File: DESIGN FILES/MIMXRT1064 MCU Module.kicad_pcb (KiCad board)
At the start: 6 copper layers, 60 x 22 mm, 74 parts, among them J601 TF-15x15, U401 MIMXRT1064CVL5B, U601 IS25WP064A-JBLE, U602 IS42S16160J-6BLI, U701 M.2-B-KEY, Y401 7V24000026, Y402 Q13FC1350000200

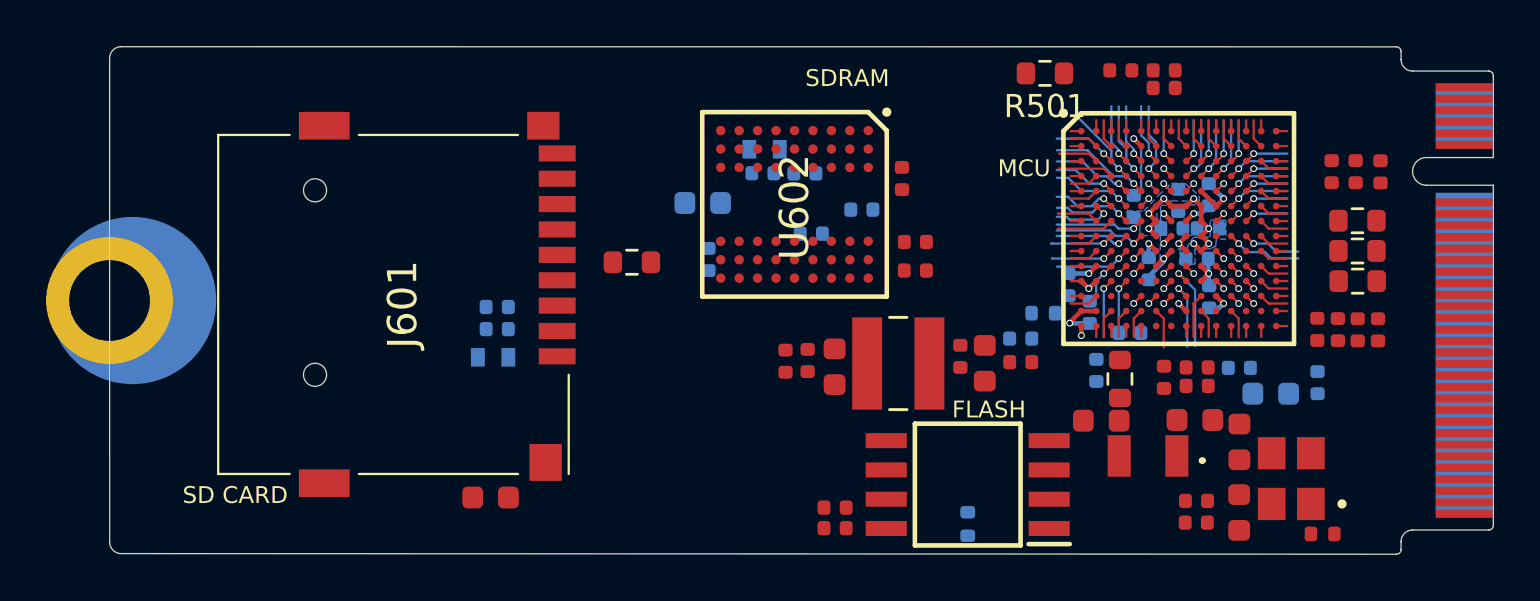
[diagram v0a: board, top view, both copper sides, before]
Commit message: updates
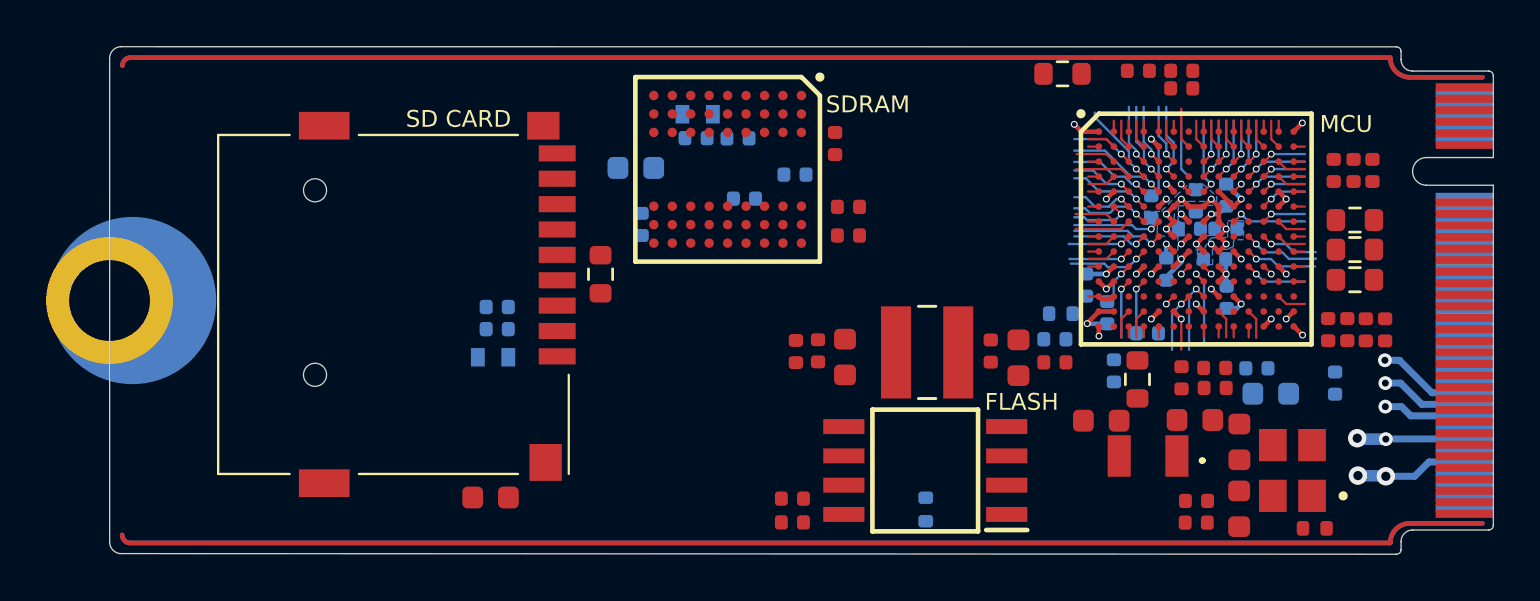
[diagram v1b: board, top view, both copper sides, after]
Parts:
- moved C602 3.27 mm to (144.3, 95.7)
- moved C601 3.27 mm to (141.7, 97.0)
- moved C603 3.27 mm to (150.3, 95.9)
- moved C605 3.27 mm to (150.9, 98.7)
- moved C609 3.27 mm to (150.9, 99.9)
- moved C611 3.27 mm to (141.9, 99.5)
- moved U602 3.27 mm to (145.6, 97.1)
- moved C604 3.27 mm to (146.1, 95.7)
- moved C607 3.27 mm to (148.6, 97.3)
- moved C610 3.27 mm to (146.4, 98.3)
- moved FB601 3.27 mm to (144.3, 94.7)
- moved U601 1.94 mm to (154.2, 110.1)
- moved R601 1.93 mm to (154.2, 111.8)
- moved C606 1.89 mm to (148.4, 111.3)
- moved C608 1.87 mm to (148.4, 112.4)
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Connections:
- net Net-(R501-Pad1) renamed /MCU GPIO & BUS/SDRAM_CLK_RES
- net Net-(R502-Pad1) renamed /MCU GPIO & BUS/SD_CLK_RES
- net Net-(R503-Pad1) renamed /MCU GPIO & BUS/FLEXSPI_CLK_RES
- net Net-(R504-Pad2) renamed /MCU GPIO & BUS/I2S_MCLK_RES
- net Net-(R505-Pad2) renamed /MCU GPIO & BUS/I2S_BCLK_RES
- net Net-(R506-Pad2) renamed /MCU GPIO & BUS/I2C_LRC_RES
- U401 pad J5: /MCU POWER & CRYSTALS/VDD_SOC_IN -> unconnected-(U401-PadJ5)
- U701 pad P$62: +5V -> VBUS
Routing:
- net GND: track 31.4 -> 20.8 mm, vias 12 -> 18
- net /MCU POWER & CRYSTALS/VDD_SOC_IN: track 14.7 -> 7.22 mm, vias 8 -> 7
- net +1V8: track 0.45 -> 7.88 mm, vias 1 -> 4
- net VBUS: track 1.71 -> 6.49 mm, vias 0 -> 3
- net SD_CMD: track 0.00 -> 3.49 mm, vias 0 -> 1
- net PMIC_ON_REQ: track 0.45 -> 3.88 mm
- net /MCU GPIO & BUS/USB CAP: track 0.45 -> 3.87 mm
- net JTAG_nTRST: track 0.45 -> 3.34 mm
- net IO2: track 0.45 -> 3.33 mm
- net SPI_SOUT: track 0.45 -> 3.33 mm
- net SDRAM_D2: track 3.51 -> 6.38 mm
- net SDRAM_D15: track 3.53 -> 6.41 mm
- net SDRAM_D13: track 7.26 -> 4.39 mm
- net SDRAM_D5: track 6.74 -> 3.87 mm
- net SDRAM_D3: track 3.46 -> 6.34 mm
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- added copper zone on In3.Cu, net +1V8
- added copper zone on In3.Cu, net +3V3
- added copper zone on In1.Cu, net GND
- added copper zone on In4.Cu, net GND
- added copper zone on In3.Cu, net VBUS
